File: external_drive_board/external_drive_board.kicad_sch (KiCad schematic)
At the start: 33 parts, among them J1 MD-90SM, J2 MD-90SM, J3 Conn_02x17_Odd_Even, J4 Conn_01x04, J5 Conn_01x03, J7 Conn_01x03, SW1 SW_DIP_x04, U1 74LS125, U2 74LS85, U3 74LS595, U4 74LS165, U5 74LS04, U6 74LS165

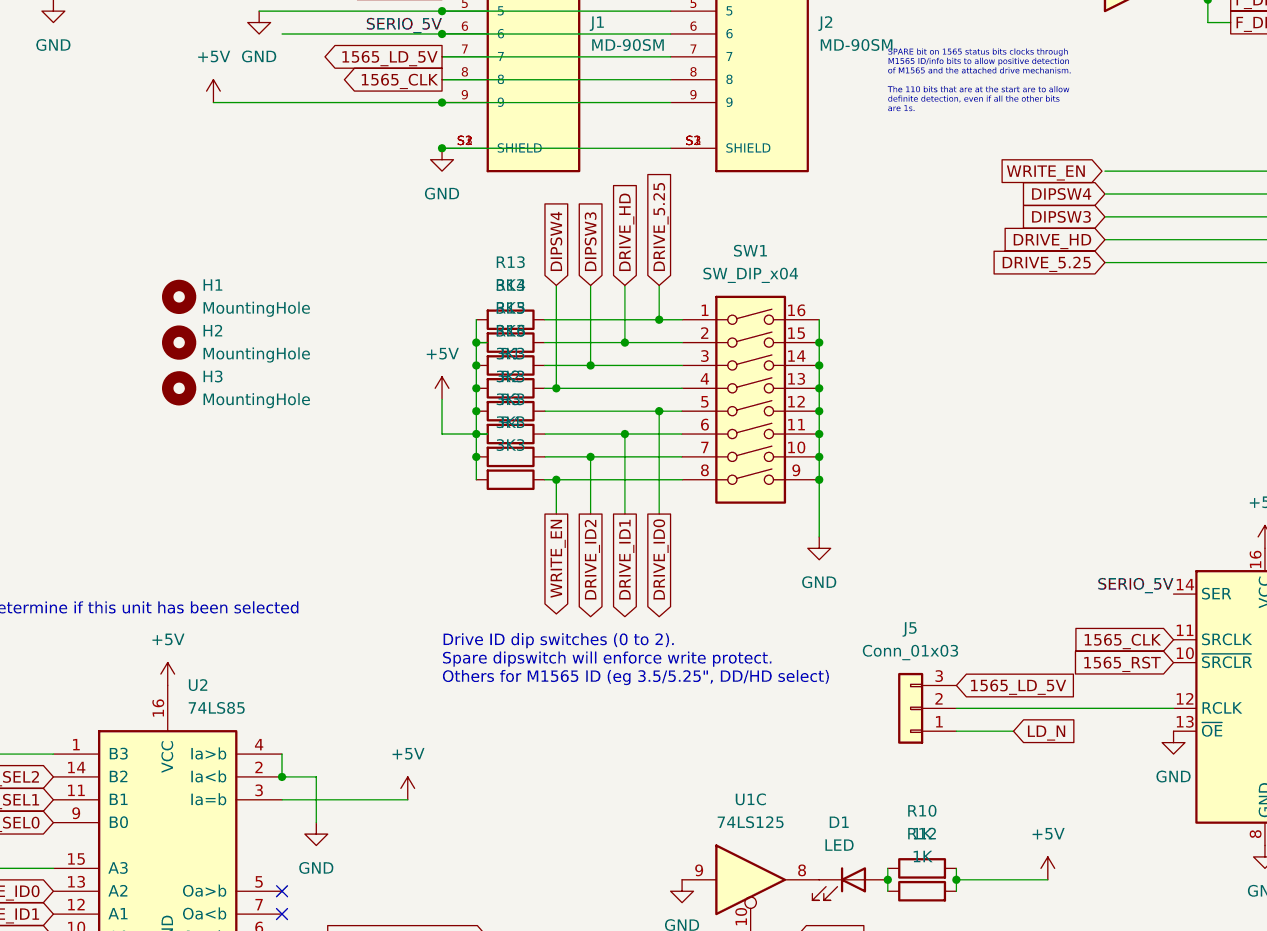
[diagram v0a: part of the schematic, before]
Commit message: finish M1565 initial board rev
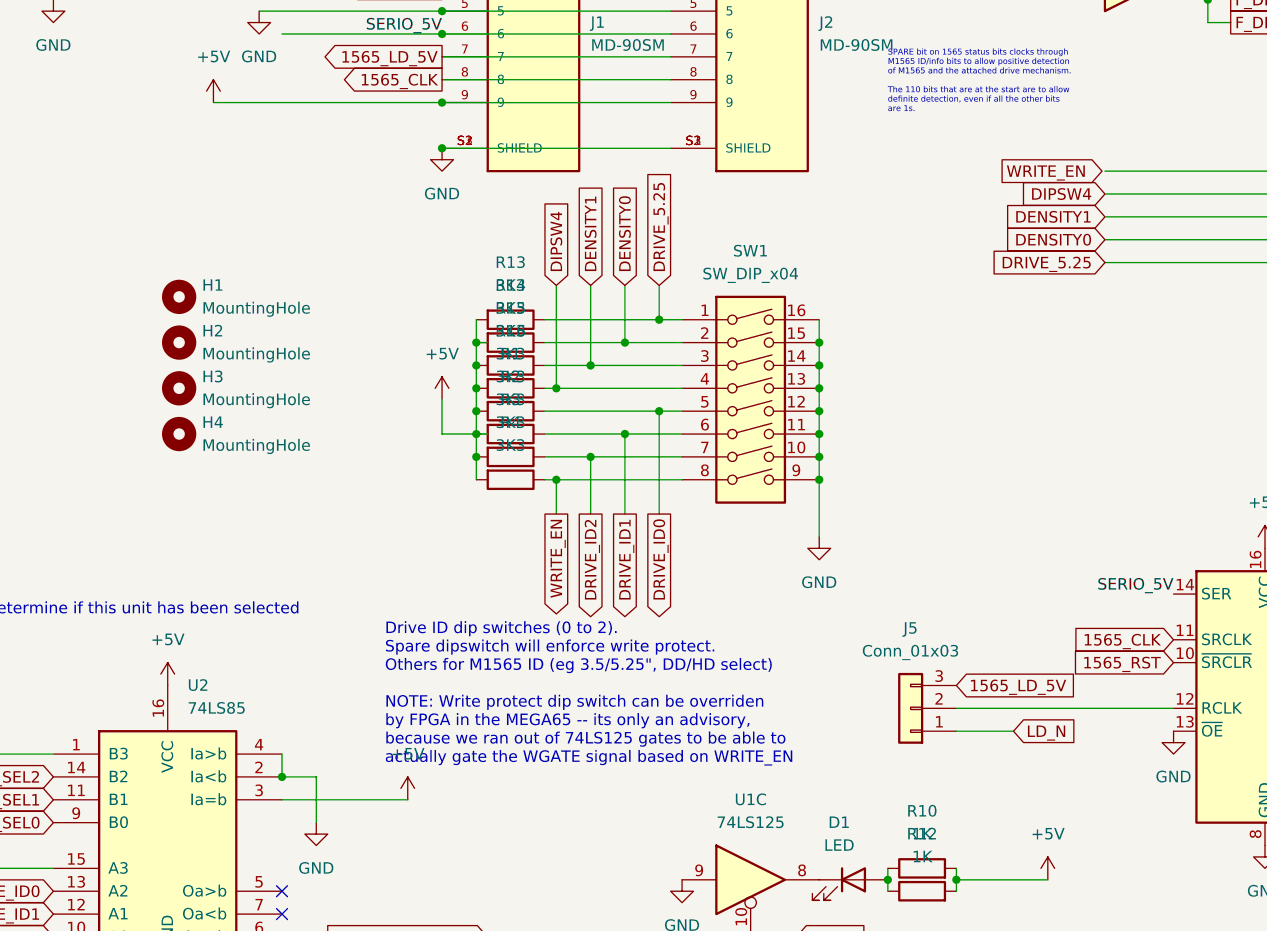
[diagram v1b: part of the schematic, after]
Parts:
- added H4: MountingHole, MountingHole:MountingHole_3mm_Pad, symbol Mechanical:MountingHole
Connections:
- net DIPSW3 renamed DENSITY1
- net DRIVE_HD renamed DENSITY0
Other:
- note added: "Drive ID dip switches (0 to 2). Spare dipswitch will enforce write protect. Others for M1565 ID (eg 3.5/5.25", DD/HD select) NOTE: Write protect dip switch can be overriden by FPGA in the MEGA65 -- its only an advisory, because we ran out of 74LS125 gates to be able to actually gate the WGATE signal based on WRITE_EN"
- note removed: "Drive ID dip switches (0 to 2). Spare dipswitch will enforce write protect. Others for M1565 ID (eg 3.5/5.25", DD/HD select)"
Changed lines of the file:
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@@
     (effects (font (size 1.27 1.27)) (justify left bottom))
   )
-  (text "Drive ID dip switches (0 to 2).\nSpare dipswitch will enforce write protect.\nOthers for M1565 ID (eg 3.5/5.25\", DD/HD select)"
-    (at 73.66 123.19 0)
+  (text "Drive ID dip switches (0 to 2).\nSpare dipswitch will enforce write protect.\nOthers for M1565 ID (eg 3.5/5.25\", DD/HD select)\n\nNOTE: Write protect dip switch can be overriden\nby FPGA in the MEGA65 -- its only an advisory,\nbecause we ran out of 74LS125 gates to be able to\nactually gate the WGATE signal based on WRITE_EN"
+    (at 67.31 132.08 0)
     (effects (font (size 1.27 1.27)) (justify left bottom))
   )
@@
     )
   )
-  (global_label "DIPSW3" (shape input) (at 147.32 71.12 180) (fields_autoplaced)
-    (effects (font (size 1.27 1.27)) (justify right))
-    (property "Intersheetrefs" "${INTERSHEET_REFS}" (at 137.3196 71.12 0)
+  (global_label "DENSITY1" (shape input) (at 147.32 71.12 180) (fields_autoplaced)
+    (effects (font (size 1.27 1.27)) (justify right))
+    (property "Intersheetrefs" "${INTERSHEET_REFS}" (at 135.5053 71.12 0)
       (effects (font (size 1.27 1.27)) (justify right) hide)
     )
@@
     )
   )
-  (global_label "DRIVE_HD" (shape input) (at 93.98 78.74 90) (fields_autoplaced)
-    (effects (font (size 1.27 1.27)) (justify left))
-    (property "Intersheetrefs" "${INTERSHEET_REFS}" (at 93.98 66.8043 90)
+  (global_label "DENSITY0" (shape input) (at 93.98 78.74 90) (fields_autoplaced)
+    (effects (font (size 1.27 1.27)) (justify left))
+    (property "Intersheetrefs" "${INTERSHEET_REFS}" (at 93.98 66.9253 90)
       (effects (font (size 1.27 1.27)) (justify left) hide)
     )
@@
     )
   )
-  (global_label "DIPSW3" (shape input) (at 90.17 78.74 90) (fields_autoplaced)
-    (effects (font (size 1.27 1.27)) (justify left))
-    (property "Intersheetrefs" "${INTERSHEET_REFS}" (at 90.17 68.7396 90)
+  (global_label "DENSITY1" (shape input) (at 90.17 78.74 90) (fields_autoplaced)
+    (effects (font (size 1.27 1.27)) (justify left))
+    (property "Intersheetrefs" "${INTERSHEET_REFS}" (at 90.17 66.9253 90)
       (effects (font (size 1.27 1.27)) (justify left) hide)
     )
@@
     )
   )
-  (global_label "DRIVE_HD" (shape input) (at 147.32 73.66 180) (fields_autoplaced)
-    (effects (font (size 1.27 1.27)) (justify right))
-    (property "Intersheetrefs" "${INTERSHEET_REFS}" (at 135.3843 73.66 0)
+  (global_label "DENSITY0" (shape input) (at 147.32 73.66 180) (fields_autoplaced)
+    (effects (font (size 1.27 1.27)) (justify right))
+    (property "Intersheetrefs" "${INTERSHEET_REFS}" (at 135.5053 73.66 0)
       (effects (font (size 1.27 1.27)) (justify right) hide)
     )
@@
         )
       )
+    )
+  )
+  (symbol (lib_id "Mechanical:MountingHole") (at 44.45 95.25 0) (unit 1)
+    (in_bom yes) (on_board yes) (dnp no) (fields_autoplaced)
+    (property "Reference" "H4" (at 46.99 93.98 0)
+      (effects (font (size 1.27 1.27)) (justify left))
+    )
+    (property "Value" "MountingHole" (at 46.99 96.52 0)
+      (effects (font (size 1.27 1.27)) (justify left))
+    )
+    (property "Footprint" "MountingHole:MountingHole_3mm_Pad" (at 44.45 95.25 0)
+      (effects (font (size 1.27 1.27)) hide)
+    )
+    (property "Datasheet" "~" (at 44.45 95.25 0)
+      (effects (font (size 1.27 1.27)) hide)
+    )
+    (instances
+      (project "external_drive_board"
+        (path "/0105c347-4e24-4e51-91e8-df67c5985c25"
+          (reference "H4") (unit 1)
+        )
+      )
